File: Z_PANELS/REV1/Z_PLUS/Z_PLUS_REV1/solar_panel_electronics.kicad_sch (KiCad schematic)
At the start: 18 parts, among them U2 LTC3130EUDC-1-PBF

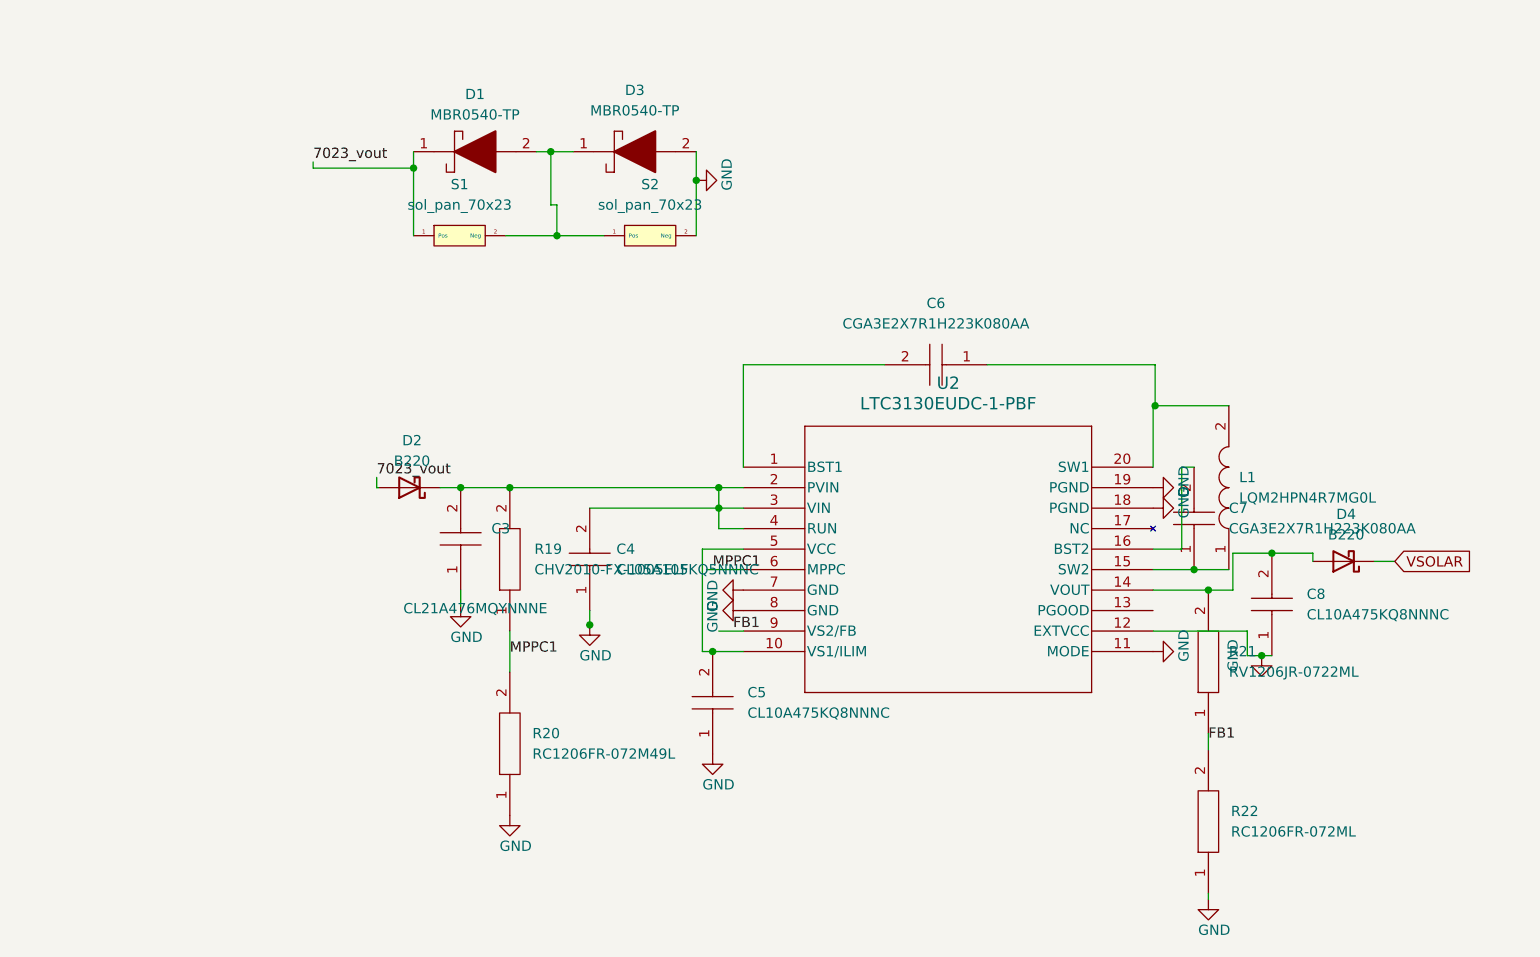
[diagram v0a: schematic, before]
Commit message: made changes to Z plus board
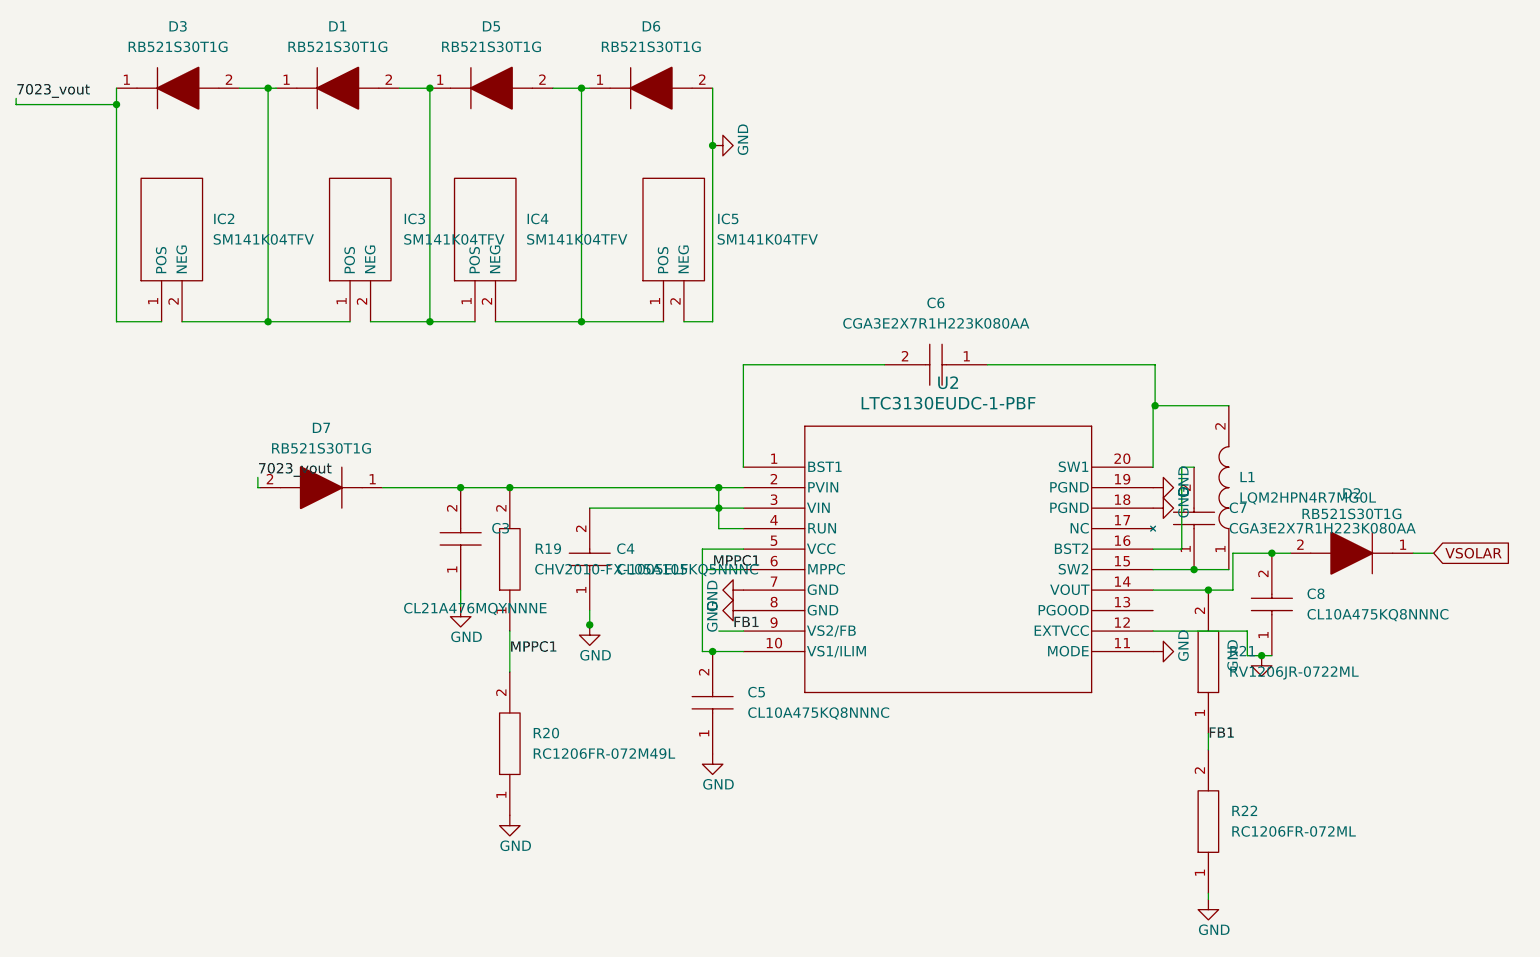
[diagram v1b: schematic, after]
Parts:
- removed D1, D3: MBR0540-TP, SOD3716X135N, symbol AA_AUTO_LOADER:MBR0540-TP
- removed D2, D4: B220, Diode_SMD:D_SMB, symbol Diode:B220
- removed S1, S2: sol_pan_70x23, CUSTOM_SOLAR_7023:sol_pan_SM141K10TFS_70x23, symbol solar_symbol_lib:sol_pan_70x23
- added D1, D2, D3, D5, D6, D7: RB521S30T1G, SODFL1608X70N, symbol AA_AUTO_LOADER:RB521S30T1G
- added IC2, IC3, IC4, IC5: SM141K04TFV, SODFL490150X120N, symbol AA_AUTO_LOADER:SM141K04TFV
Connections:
- net 7023_vout: now also D3.1, D7.2, IC2.1 (POS)
- net GND: now also D6.2, IC5.2 (NEG)
- net VSOLAR: now also D2.1
- net at C8.2, R21.2, U2.14 (VOUT): now also D2.2
- net at C3.2, C4.2, R19.2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: now also D7.1
- new net: D1.1, D3.2, IC2.2 (NEG), IC3.1 (POS)
- new net: D1.2, D5.1, IC3.2 (NEG), IC4.1 (POS)
- new net: D5.2, D6.1, IC4.2 (NEG), IC5.1 (POS)
